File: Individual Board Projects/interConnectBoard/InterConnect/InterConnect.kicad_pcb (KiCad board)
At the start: 2 copper layers, 14.5 x 30 mm, 2 parts, among them J1 5x2.54mm+2xBus, J2 5x2.54mm+2xBus

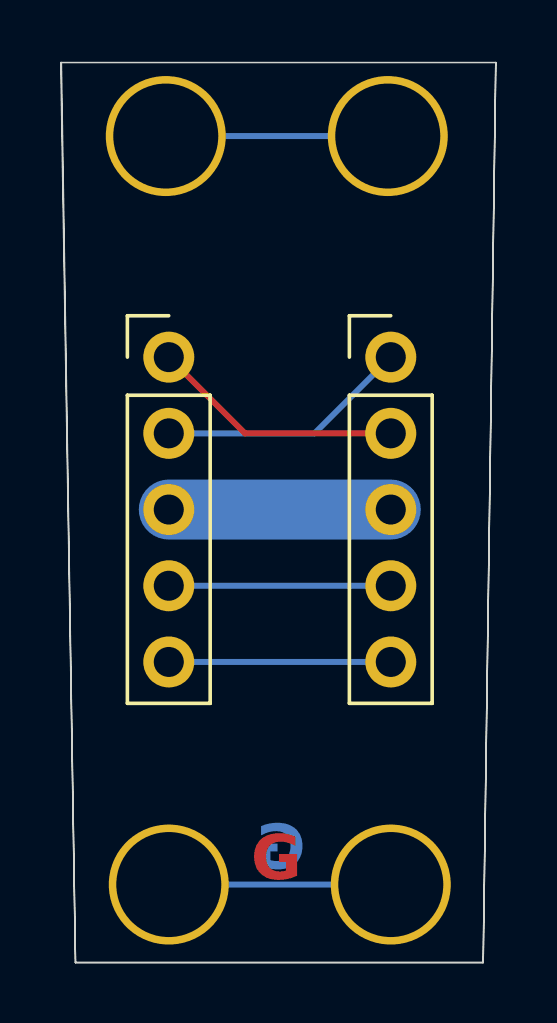
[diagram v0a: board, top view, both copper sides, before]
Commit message: Controll Finished - READY TO FAB
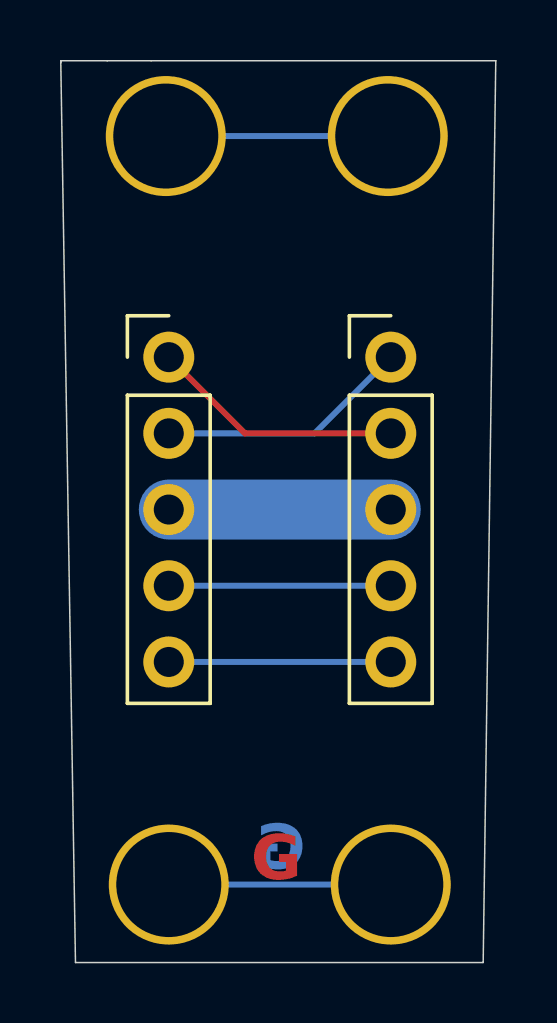
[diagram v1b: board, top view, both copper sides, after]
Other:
- board size 14.5 x 30 mm -> 14.5 x 30.1 mm
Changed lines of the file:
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@@
 	)
 	(gr_line
-		(start 122.45 85.1)
-		(end 136.95 85.1)
-		(stroke
-			(width 0.05)
-			(type default)
-		)
-		(layer "Edge.Cuts")
-	)
-	(gr_line
-		(start 136.95 85.1)
+		(start 136.95 85.04)
 		(end 136.53 115.1)
 		(stroke
@@
 	)
 	(gr_line
-		(start 136.53 115.1)
-		(end 122.94 115.1)
+		(start 122.44902 85.04)
+		(end 122.45 85.1)
 		(stroke
 			(width 0.05)
@@
 	)
 	(gr_line
-		(start 122.94 115.1)
-		(end 122.47 85.1)
+		(start 125.46 85.04)
+		(end 136.95 85.04)
 		(stroke
 			(width 0.05)
@@
 	)
 	(gr_line
-		(start 136.95 85.1)
-		(end 136.53 115.1)
+		(start 125.46 85.04)
+		(end 124 85.04)
+		(stroke
+			(width 0.05)
+			(type default)
+		)
+		(layer "Edge.Cuts")
+	)
+	(gr_line
+		(start 124 85.04)
+		(end 122.44902 85.04)
 		(stroke
 			(width 0.05)
@@
 		)
 	)
+	(dimension
+		(type orthogonal)
+		(layer "Eco2.User")
+		(pts
+			(xy 125.96 86.82) (xy 125.96 84.31)
+		)
+		(height -20.14)
+		(orientation 1)
+		(format
+			(prefix "")
+			(suffix "")
+			(units 3)
+			(units_format 0)
+			(precision 4)
+			(suppress_zeroes yes)
+		)
+		(style
+			(thickness 0.1)
+			(arrow_length 1.27)
+			(text_position_mode 0)
+			(arrow_direction outward)
+			(extension_height 0.58642)
+			(extension_offset 0.5)
+			(keep_text_aligned yes)
+		)
+		(gr_text "2.51"
+			(at 104.67 85.565 90)
+			(layer "Eco2.User")
+			(effects
+				(font
+					(size 1 1)
+					(thickness 0.15)
+				)
+			)
+		)
+	)
